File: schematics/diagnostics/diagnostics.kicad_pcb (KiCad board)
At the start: 2 copper layers, 30.5 x 17.8 mm, 12 parts, among them J2 Conn_01x06_Socket, J3 Conn_02x04_Odd_Even, U1 CH340N

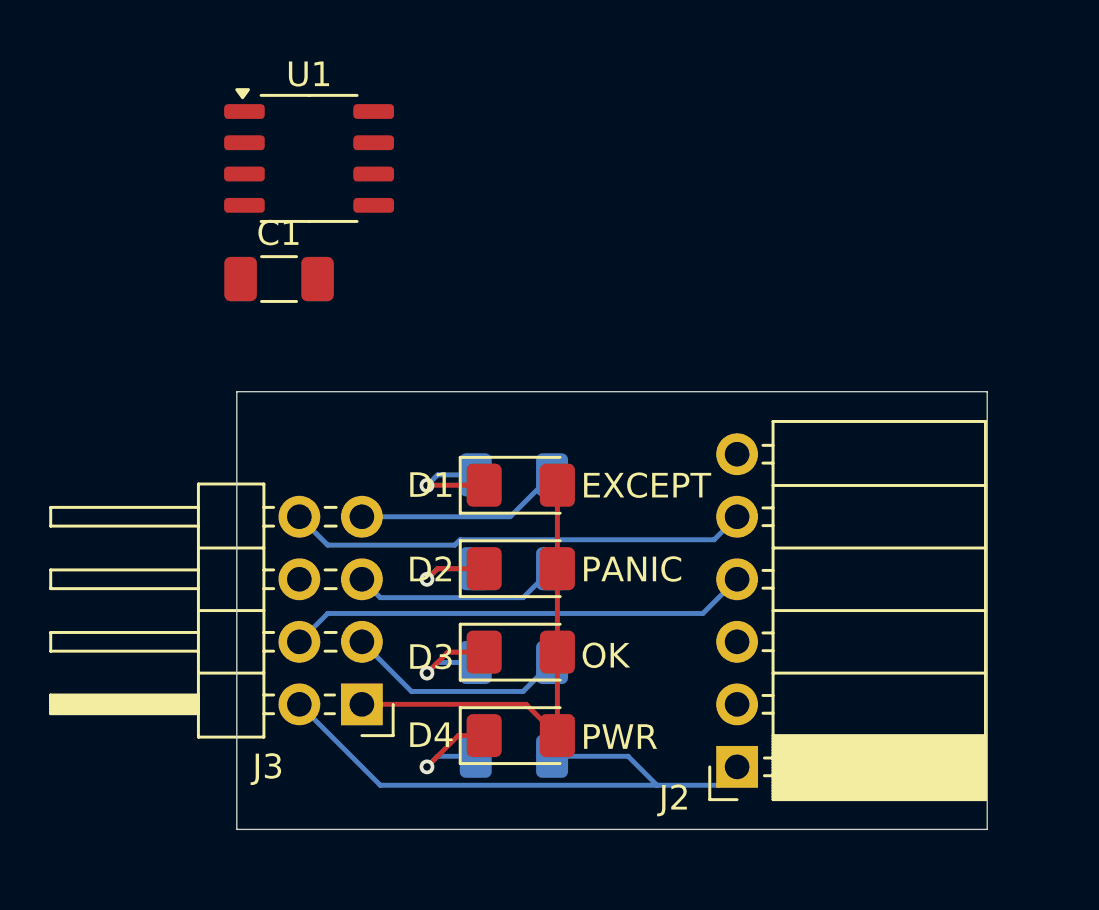
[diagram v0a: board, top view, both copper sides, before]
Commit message: Signed-off-by: Ray33ee <30669752+ray33ee@users.noreply.github.com>
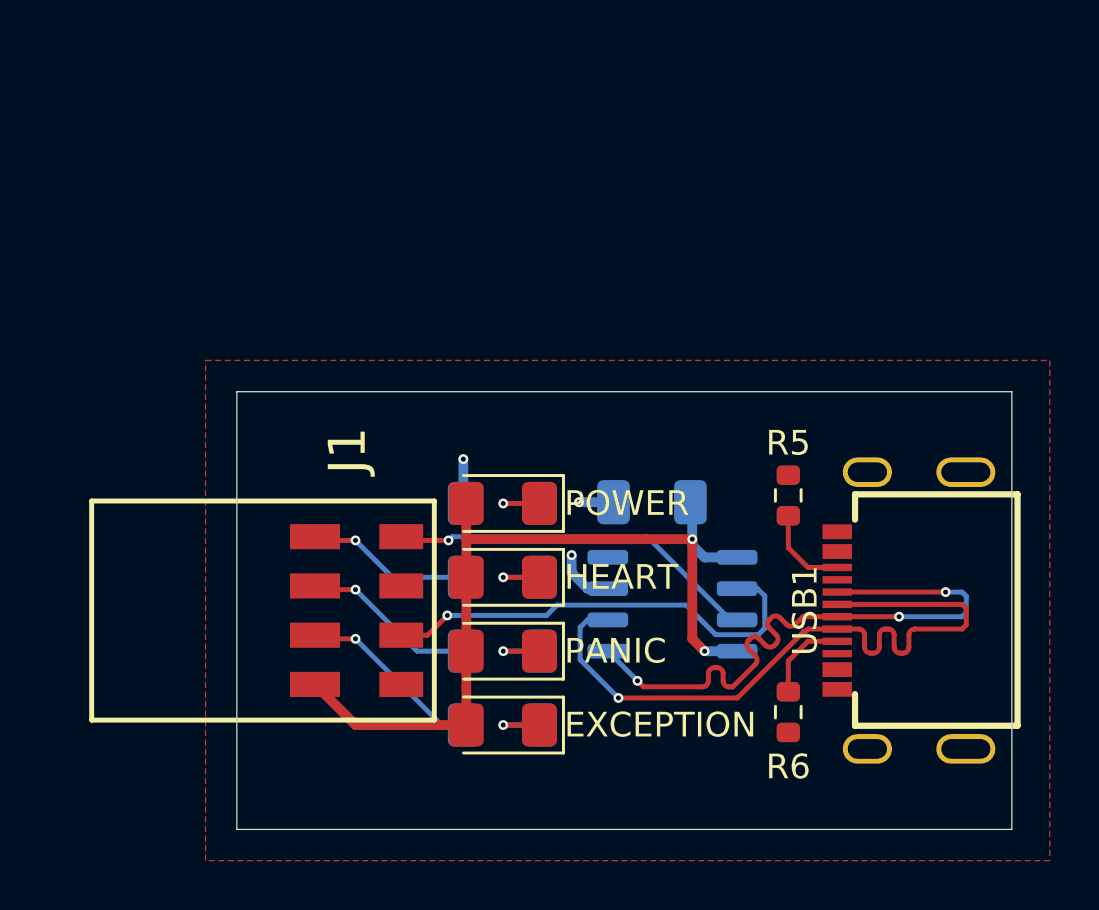
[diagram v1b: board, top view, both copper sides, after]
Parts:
- removed J2: Conn_01x06_Socket, Connector_PinSocket_2.54mm:PinSocket_1x06_P2.54mm_Horizontal
- removed J3: Conn_02x04_Odd_Even, Connector_PinHeader_2.54mm:PinHeader_2x04_P2.54mm_Horizontal
- added J1: SAMTEC-MMT-104-02-X-DH, custom:SAMTEC-MMT-104-02-X-DH, F.Cu at (118.1, 88.9)
- added R5: 0603WAF5101T5E, Resistor_SMD:R_0603_1608Metric, F.Cu at (140.5, 84.2)
- added R6: 0603WAF5101T5E, Resistor_SMD:R_0603_1608Metric, F.Cu at (140.5, 93.0)
- added USB1: TYPE-C-31-M-13, custom:USB-C-SMD_TYPE-C-31-M-13, F.Cu at (145.1, 88.9)
- C1, U1: moved to B.Cu
- moved U1 23.4 mm to (135.8, 88.6)
- moved C1 17.7 mm to (135.0, 84.5), turned to 180 degrees
- moved R4 10.3 mm to (128.9, 84.5), turned to 0 degrees
- moved R1 10.2 mm to (128.9, 93.5), turned to 0 degrees
- moved D1 9.77 mm to (128.9, 93.5), turned to 180 degrees
- moved D4 9.46 mm to (128.9, 84.5), turned to 180 degrees
- moved R3 3.49 mm to (128.9, 87.5), turned to 0 degrees
- moved D2 3.43 mm to (128.9, 90.5), turned to 180 degrees
- moved R2 3.38 mm to (128.9, 90.5), turned to 0 degrees
- moved D3 3.13 mm to (128.9, 87.5), turned to 180 degrees
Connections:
- net Net-(D1-K) renamed /EXC
- net Net-(D2-K) renamed /PAN
- net Net-(D3-K) renamed /BEAT
- net Net-(D4-K) renamed /PWR
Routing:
- net D-: track 0.00 -> 29.1 mm, vias 0 -> 1
- net D+: track 0.00 -> 26.1 mm, vias 0 -> 3
- net GND: track 24.2 -> 5.67 mm, vias 0 -> 3
- net +3V3: track 18.6 -> 35.5 mm, vias 0 -> 2
- net Net-(USB1-CC2): track 0.00 -> 3.62 mm
- net Net-(USB1-CC1): track 0.00 -> 3.57 mm
- net RX: track 18.7 -> 15.2 mm, vias 0 -> 1
- net HEART: track 9.05 -> 6.73 mm, vias 0 -> 1
- net /PWR: track 5.01 -> 2.97 mm
- net /BEAT: track 4.83 -> 2.97 mm
- net /PAN: track 4.66 -> 2.97 mm
- net /EXC: track 4.48 -> 2.97 mm
- net PANIC: track 8.52 -> 7.14 mm, vias 0 -> 1
- net EXCEPTION: track 8.43 -> 7.56 mm, vias 0 -> 1
- net TX: track 18.8 -> 18.4 mm, vias 0 -> 1
- added copper zone on F.Cu, net GND
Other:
- board size 30.5 x 17.8 mm -> 31.5 x 17.8 mm
- board text added: "EXCEPTION"
- board text added: "HEART"
- board text added: "POWER"
- board text removed: "EXCEPT"
- board text removed: "OK"
- board text removed: "PWR"
